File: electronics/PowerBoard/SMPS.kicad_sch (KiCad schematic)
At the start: 12 parts, among them U201 XL1509-5.0E1

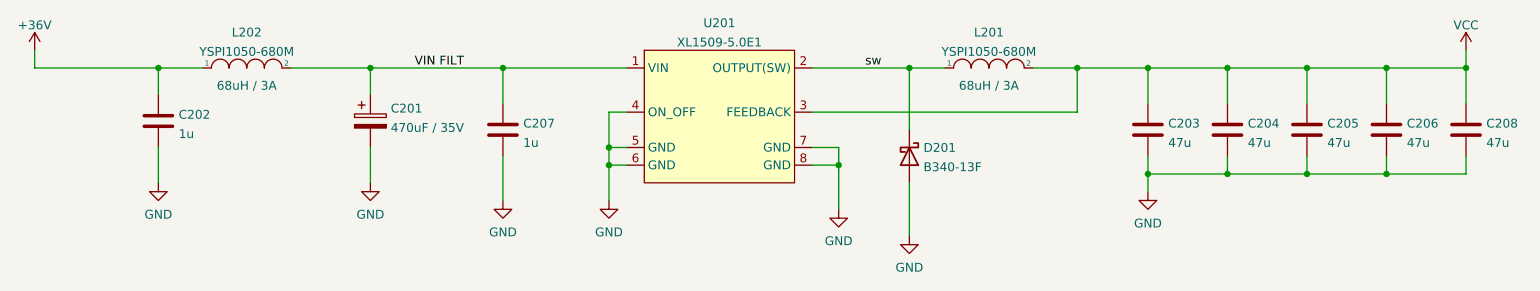
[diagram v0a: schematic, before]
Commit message: PowerBoard commit
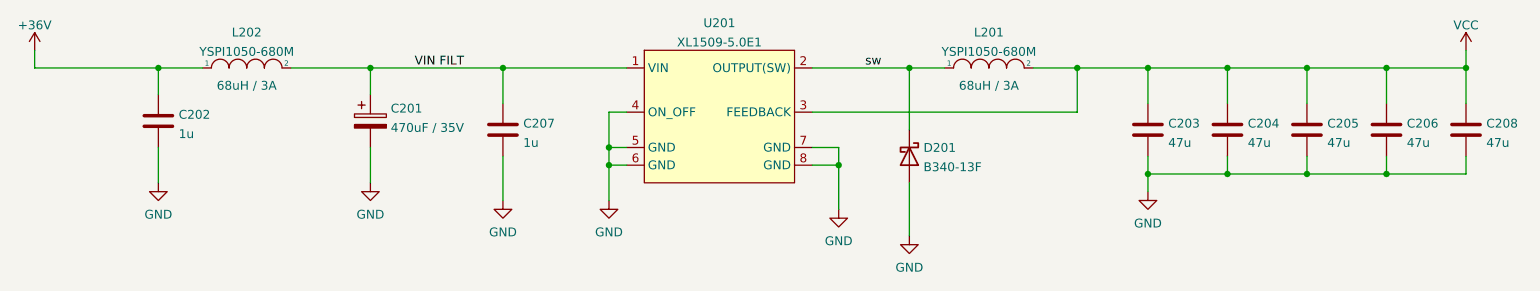
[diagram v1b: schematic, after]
